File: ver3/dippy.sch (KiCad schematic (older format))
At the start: 28 parts, among them J1 Conn_01x02_Female, J2 Screw_Terminal_01x03, J3 Screw_Terminal_01x04, J4 Conn_Coaxial, J5 Conn_02x03_Odd_Even, J6 Screw_Terminal_01x04, J7 Conn_01x02_Female, U1 ATmega328P-PU-C, U2 RFM95W-915S2, U3 MCP1700-3302E_SOT23, Y1 Crystal

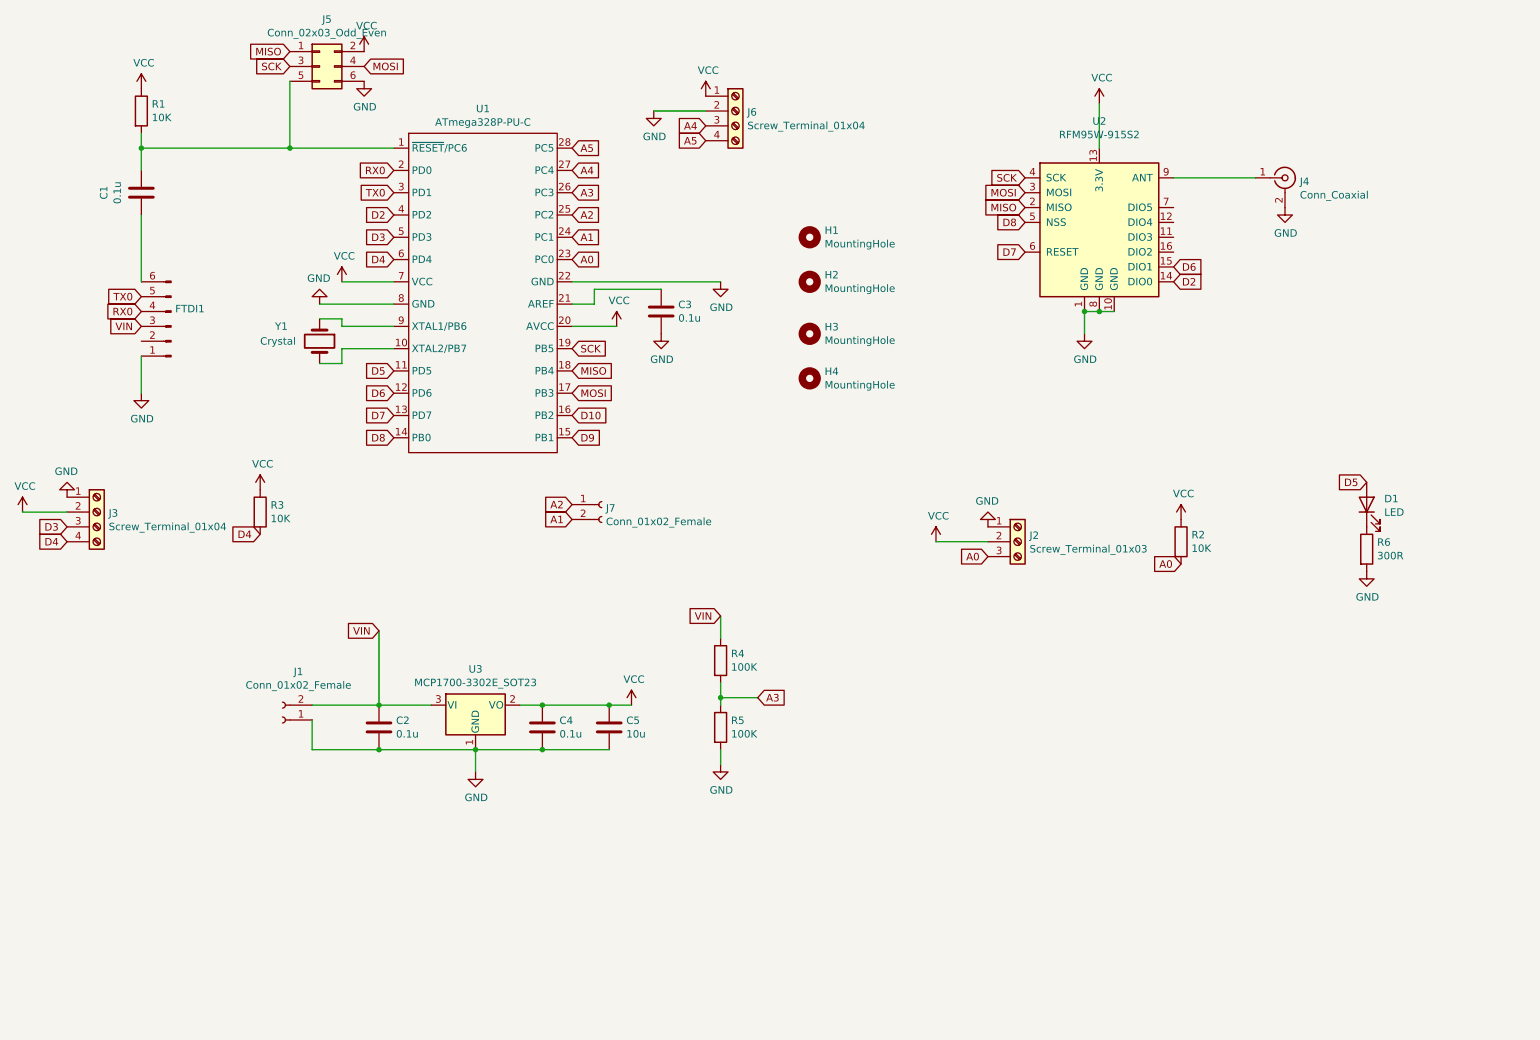
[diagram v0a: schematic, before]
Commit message: update
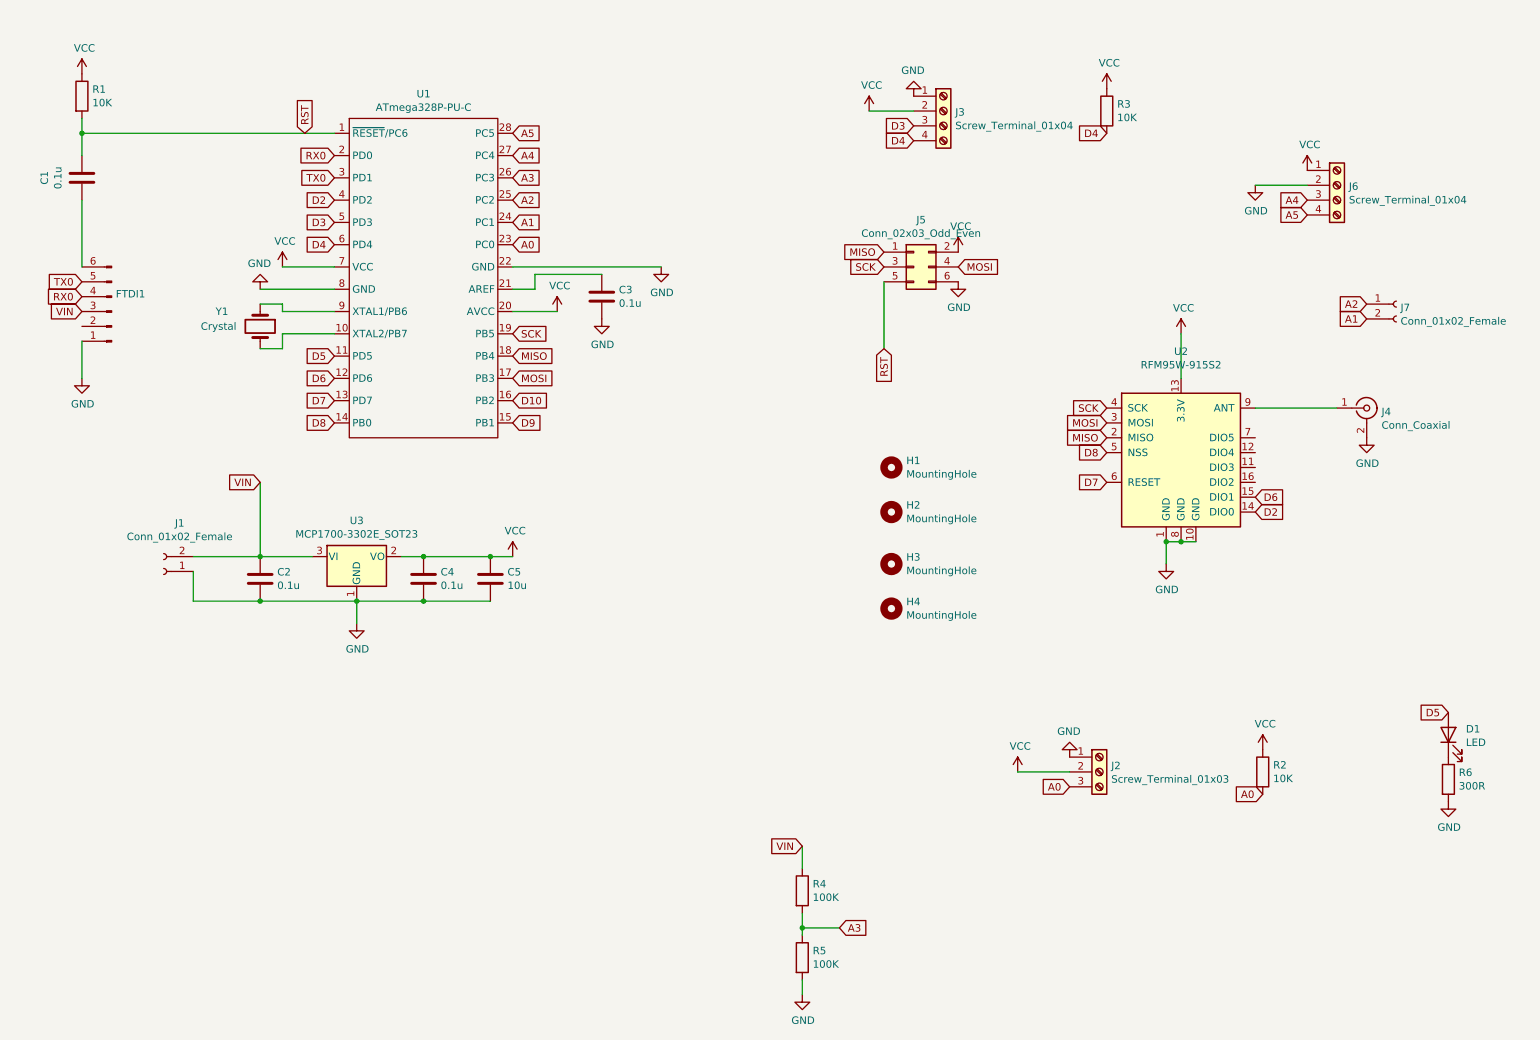
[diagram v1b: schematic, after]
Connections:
- net RST: now reaches C1.1, J5.5 (Pin_5), R1.2, U1.1 (~RESET~/PC6)
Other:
- moved on the sheet: C1, C2, C3, C4, C5, D1, FTDI1, H1, H2, H3, H4, J1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
